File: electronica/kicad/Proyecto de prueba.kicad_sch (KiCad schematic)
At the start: 12 parts, among them J1 Conn_01x02

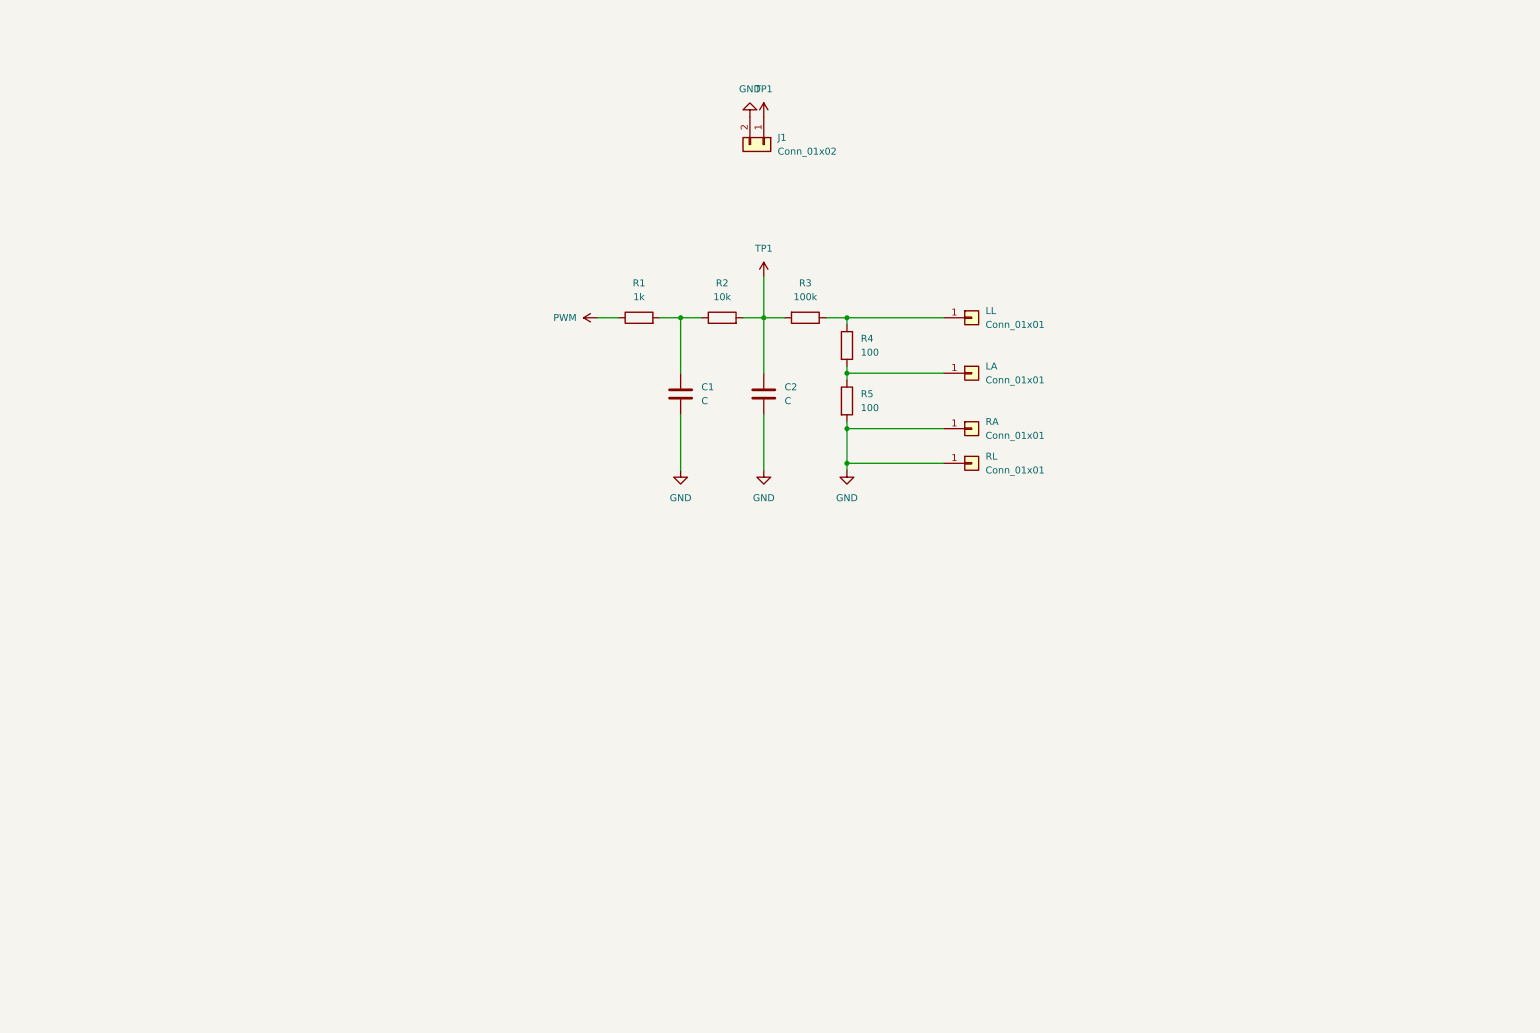
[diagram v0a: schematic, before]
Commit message: Esquematico_completado_sin_huellas
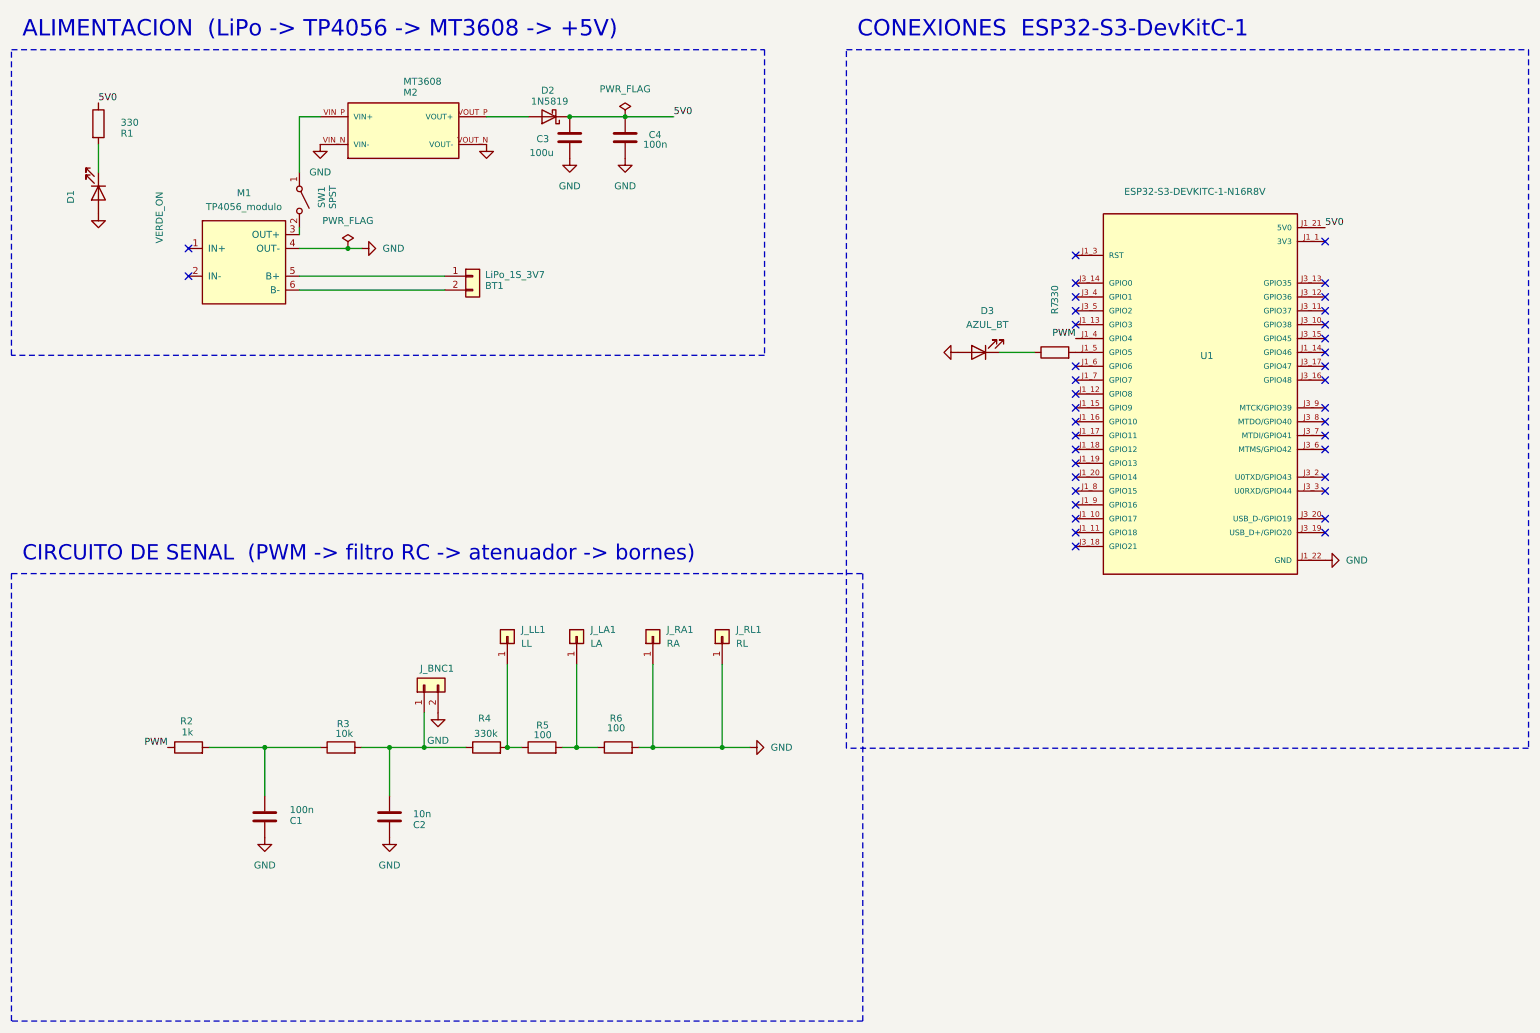
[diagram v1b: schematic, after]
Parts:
- removed J1: Conn_01x02, Connector_PinHeader_2.54mm:PinHeader_1x02_P2.54mm_Vertical, symbol Connector_Generic:Conn_01x02
- removed LA, LL, RA, RL: Conn_01x01, MountingHole:MountingHole_5mm, symbol Connector_Generic:Conn_01x01
- added BT1: LiPo_1S_3V7, symbol Connector_Generic:Conn_01x02
- added C3: 100u, symbol Device:C
- added C4: 100n, symbol Device:C
- added D1: VERDE_ON, symbol Device:LED
- added D2: 1N5819, symbol Diode:1N5819
- added D3: AZUL_BT, symbol Device:LED
- added J_BNC1: BNC, symbol Connector_Generic:Conn_01x02
- added J_LA1: LA, symbol Connector_Generic:Conn_01x01
- added J_LL1: LL, symbol Connector_Generic:Conn_01x01
- added J_RA1: RA, symbol Connector_Generic:Conn_01x01
- added J_RL1: RL, symbol Connector_Generic:Conn_01x01
- added M1: TP4056_modulo, TP4056_modulo:TP4056_modulo, symbol TP4056_modulo:TP4056_modulo
- added M2: MT3608, MT3608_DC:MT3608_DC, symbol MT3608_DC:MT3608_DC-DC_STEP_UP_CONVERTER_2A_BOOSTER_MODULE
- added R6: 100, symbol Device:R
- added R7: 330, symbol Device:R
- added SW1: SPST, symbol Switch:SW_SPST
- added U1: ESP32-S3-DEVKITC-1-N16R8V, ESP32-S3-DEVKITC-1-N16R8V:XCVR_ESP32-S3-DEVKITC-1-N16R8V, symbol ESP32-S3-DEVKITC-1-N16R8V:ESP32-S3-DEVKITC-1-N16R8V
- C1: value C -> 100n
- C2: value C -> 10n
- R1: value 1k -> 330
- R2: value 10k -> 1k
- R3: value 100k -> 10k
- R4: value 100 -> 330k
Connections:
- net GND: now also C3.1, C4.2, D1.2 (A), D3.2 (A), J_BNC1.2 (Pin_2), J_RA1.1 (Pin_1), J_RL1.1 (Pin_1), M1.4 (OUT-), M2.VIN_N (VIN-), M2.VOUT_N (VOUT-), R6.2, U1.J1_22 (GND), U1.J3_1 (GND), U1.J3_21 (GND), U1.J3_22 (GND); no longer R5.2
- net PWM: now also R2.1, U1.J1_4 (GPIO4); no longer R1.1
- net at R4.1: now also C2.1, R3.2, J_BNC1.1 (Pin_1); no longer R3.1
- net at R4.2, R5.1: now also J_LL1.1 (Pin_1)
- removed net TP1: C2.1, R2.2, R3.2
- new net: D3.1 (K), R7.1
- new net: R7.2, U1.J1_5 (GPIO5)
- new net: J_LA1.1 (Pin_1), R5.2, R6.1
- new net: D1.1 (K), R1.2
- new net: M1.3 (OUT+), SW1.2 (B)
- new net: BT1.1 (Pin_1), M1.5 (B+)
- new net: BT1.2 (Pin_2), M1.6 (B-)
- new net: M2.VIN_P (VIN+), SW1.1 (A)
- new net: D2.2 (A), M2.VOUT_P (VOUT+)
- new net: C1.1, R2.2, R3.1
- new net 3V3: U1.J1_1 (3V3), U1.J1_2 (3V3)
- new net 5V0: C3.2, C4.1, D2.1 (K), R1.1, U1.J1_21 (5V0)
- no-connect marks 0 -> 38
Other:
- note added: "ALIMENTACION (LiPo -> TP4056 -> MT3608 -> +5V)"
- note added: "CIRCUITO DE SENAL (PWM -> filtro RC -> atenuador -> bornes)"
- note added: "CONEXIONES ESP32-S3-DevKitC-1"
